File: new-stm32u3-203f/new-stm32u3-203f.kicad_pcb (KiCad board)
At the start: 6 copper layers, 14.5 x 90 mm, 82 parts, among them J1 Display, J2 SJ-3524-SMT, J3 12401826E412A, J4 Battery connector, J5 473092651, J6 UART, J7 RESET, J8 SWD, SW1 SW_SPDT, SW3 VOL+, SW4 VOL-, SW5 skip, SW6 Pause/Play, SW8 playlist/song, U1 STM32U385RGT6Q, U2 TLV320DAC3203IRGER, U4 LD39050PU33R, U5 TLV62569DBVR, U6 MCP73831T-2ACI/OT, U7 TPS63802DLAR, X1 32.768kHz

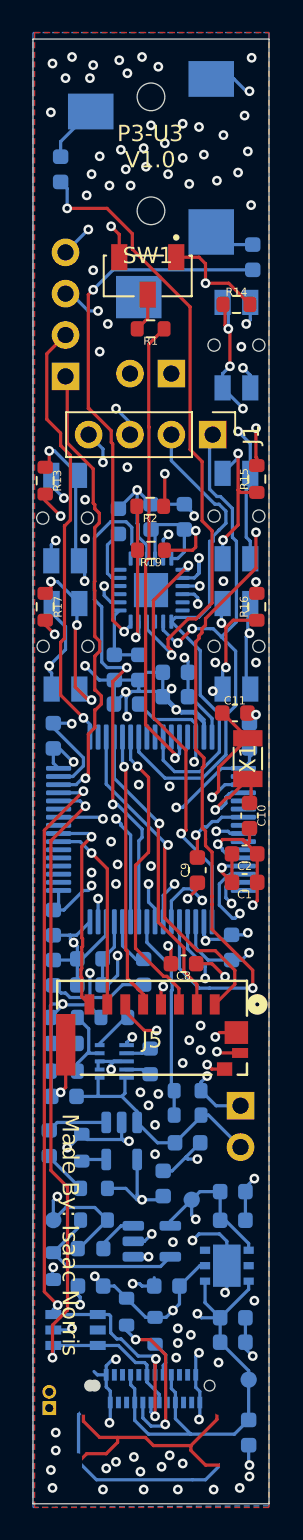
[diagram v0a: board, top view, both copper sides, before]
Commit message: finished more errors, started adding extra stuff.
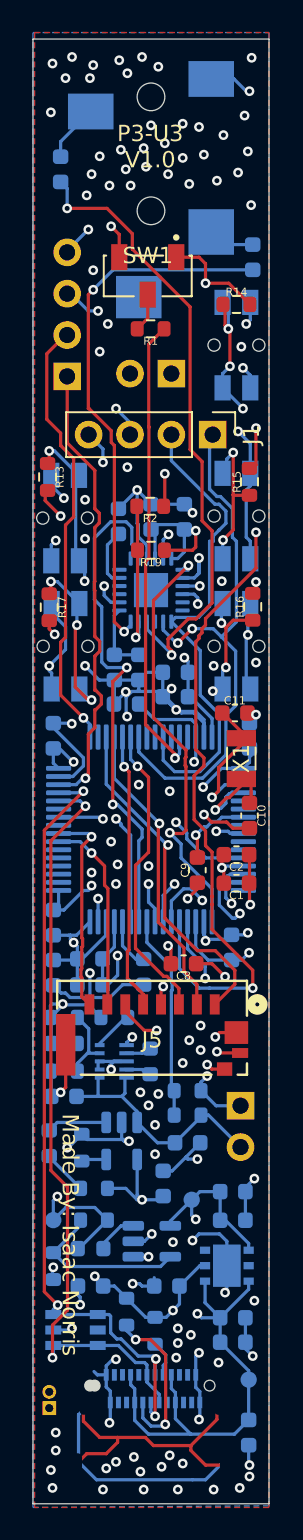
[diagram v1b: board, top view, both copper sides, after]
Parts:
- moved C1 0.50 mm to (159.5, 112.2)
- moved C2 0.50 mm to (159.5, 110.5)
- moved R15 0.48 mm to (160.3, 87.6)
- moved X1 0.40 mm to (159.8, 104.6)
- moved R13 0.27 mm to (147.9, 87.3)
- moved R17 0.25 mm to (148.0, 95.3)
- moved R16 0.25 mm to (160.5, 95.3)
- moved J8 0.10 mm to (149.1, 81.1)
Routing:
- net AVDD: track 93.3 -> 90.1 mm
- net USB_GND: track 231.3 -> 233.6 mm, vias 134 -> 135
- net MCLK_A: track 25.0 -> 26.1 mm
